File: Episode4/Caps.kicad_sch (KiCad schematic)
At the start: 192 parts

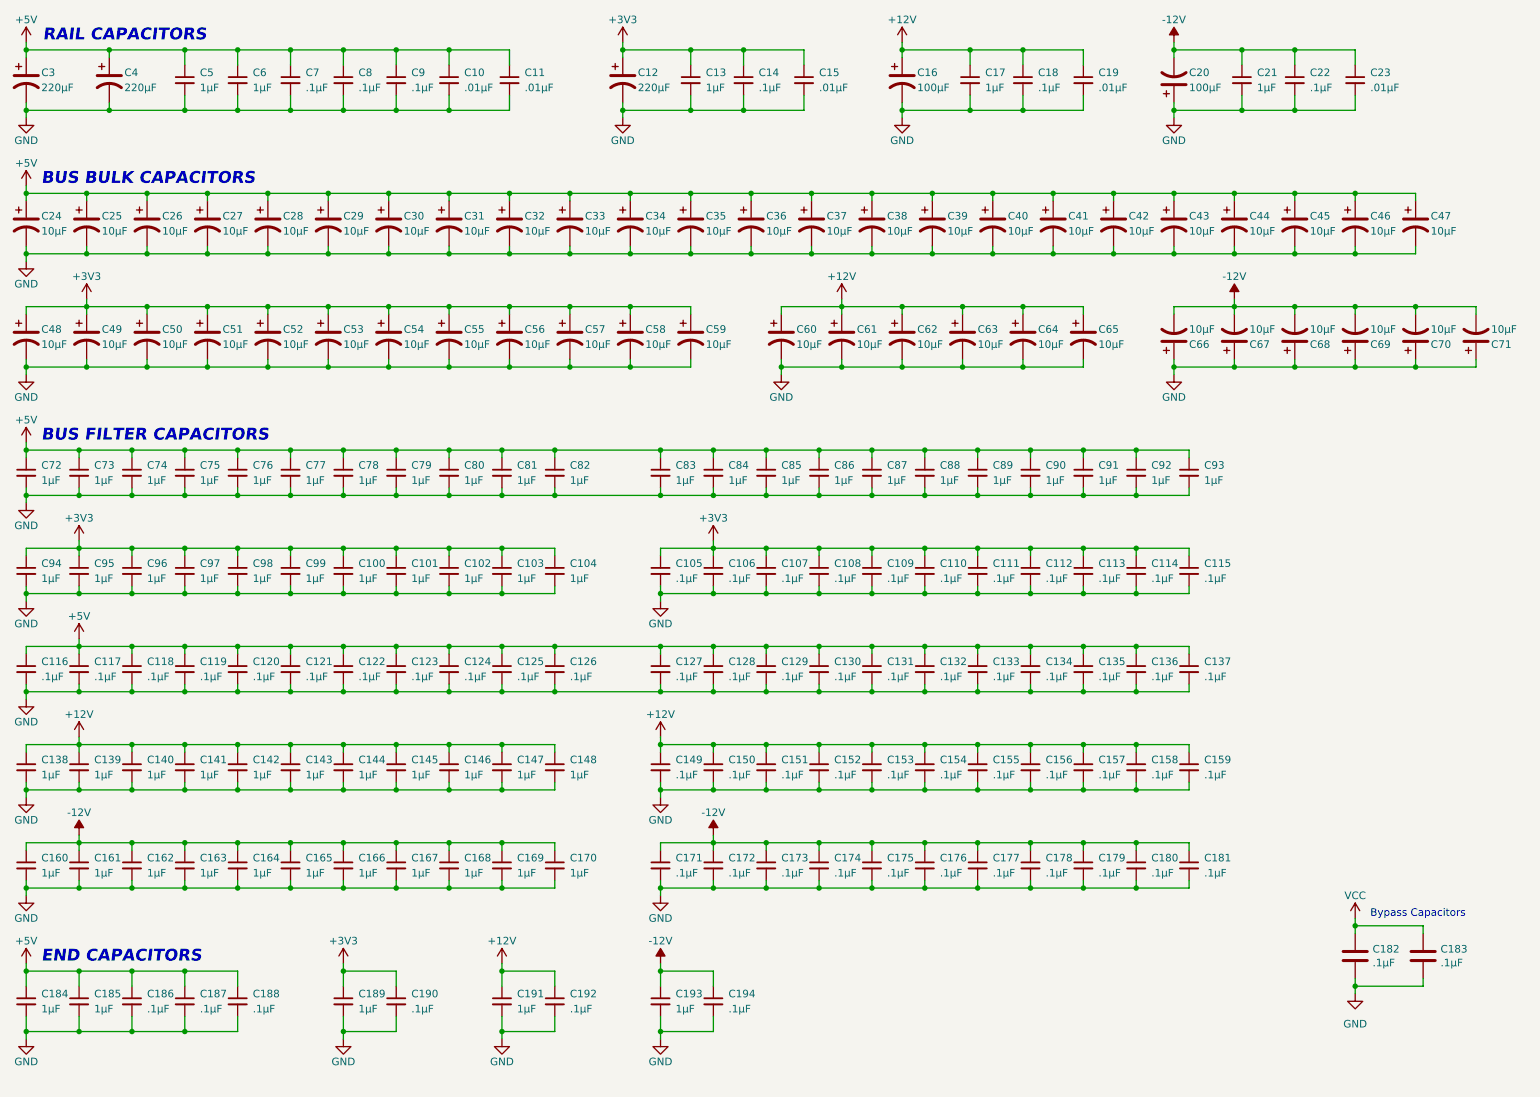
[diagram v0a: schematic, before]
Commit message: Finished the backplane
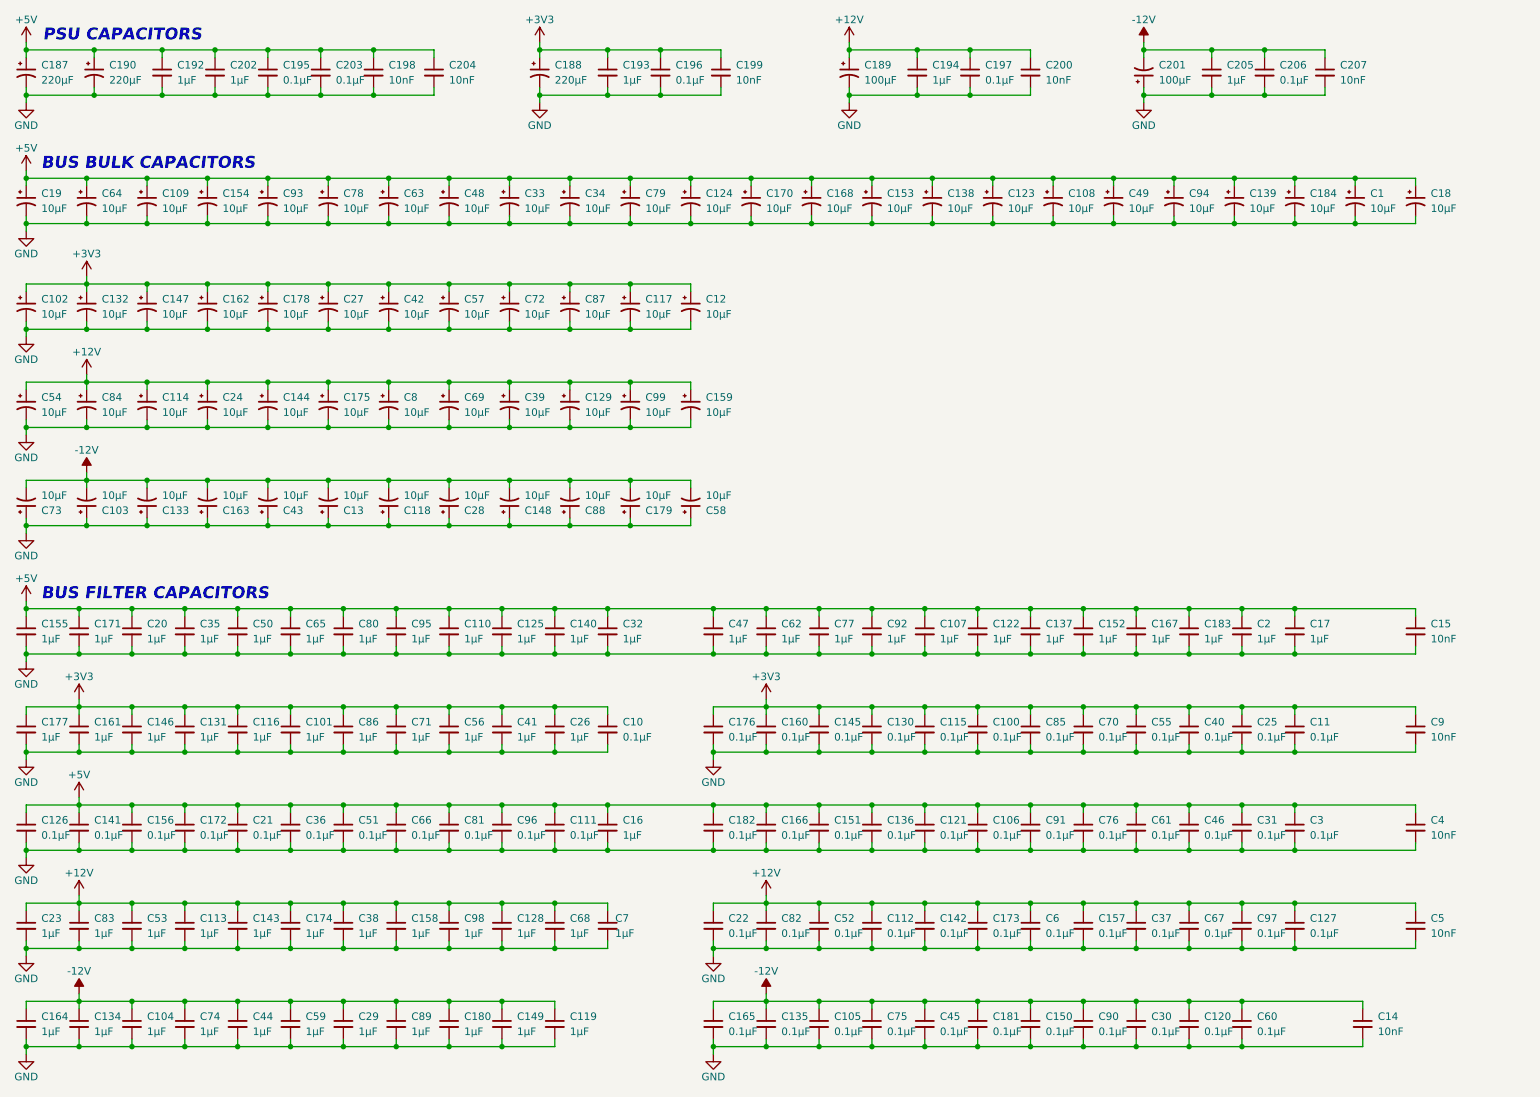
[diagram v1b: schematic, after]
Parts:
- removed C144, C145, C146, C147, C148, C165, C166, C167, C168, C169, C170, C191, C193: 1µF, Capacitor_SMD:C_0805_2012Metric_Pad1.18x1.45mm_HandSolder, symbol Device:C_Small
- removed C155, C156, C159, C171, C172, C173, C174, C175, C176, C188, C192, C194, C8: .1µF, Capacitor_SMD:C_0805_2012Metric_Pad1.18x1.45mm_HandSolder, symbol Device:C_Small
- removed C182, C183: .1µF, Capacitor_SMD:C_0805_2012Metric_Pad1.18x1.45mm_HandSolder, symbol Device:C
- added C118, C129, C148, C159, C179, C28, C39, C58, C69, C8, C88, C99: 10µF, Capacitor_SMD:CP_Elec_4x5.8, symbol Device:C_Polarized_Small_US
- added C119, C128, C149, C180, C29, C38, C59, C68, C7, C89, C98: 1µF, Capacitor_SMD:C_0805_2012Metric_Pad1.18x1.45mm_HandSolder, symbol Device:C_Small
- added C120, C127, C150, C181, C30, C37, C6, C60, C67, C90, C97: 0.1µF, Capacitor_SMD:C_0805_2012Metric_Pad1.18x1.45mm_HandSolder, symbol Device:C_Small
- added C14, C15, C4, C5, C9: 10nF, Capacitor_SMD:C_0805_2012Metric_Pad1.18x1.45mm_HandSolder, symbol Device:C_Small
- C1: renamed from C46; symbol Device:C_Polarized_US -> Device:C_Polarized_Small_US
- C10: renamed from C187; value .1µF -> 0.1µF; Manufacturer_Name Samsung Electro-Mechanics -> TAIYO YUDEN; Manufacturer_Part_Number CL21B104KBFNNNG -> MCASU21GSB7104KTNA01
- C100: renamed from C110; value .1µF -> 0.1µF; Manufacturer_Name Samsung Electro-Mechanics -> TAIYO YUDEN; Manufacturer_Part_Number CL21B104KBFNNNG -> MCASU21GSB7104KTNA01
- C101: renamed from C99; Manufacturer_Name Samsung Electro-Mechanics -> TAIYO YUDEN; Manufacturer_Part_Number CL21B105KBFNNNG -> MCASU21GSB7105KTNA01
- C102: renamed from C48; symbol Device:C_Polarized_US -> Device:C_Polarized_Small_US
- C103: renamed from C67; symbol Device:C_Polarized_US -> Device:C_Polarized_Small_US
- C104: renamed from C162; Manufacturer_Name Samsung Electro-Mechanics -> TAIYO YUDEN; Manufacturer_Part_Number CL21B105KBFNNNG -> MCASU21GSB7105KTNA01
- C105: renamed from C179; value .1µF -> 0.1µF; Manufacturer_Name Samsung Electro-Mechanics -> TAIYO YUDEN; Manufacturer_Part_Number CL21B104KBFNNNG -> MCASU21GSB7104KTNA01
- C106: renamed from C132; value .1µF -> 0.1µF; Manufacturer_Name Samsung Electro-Mechanics -> TAIYO YUDEN; Manufacturer_Part_Number CL21B104KBFNNNG -> MCASU21GSB7104KTNA01
- C107: renamed from C88; Manufacturer_Name Samsung Electro-Mechanics -> TAIYO YUDEN; Manufacturer_Part_Number CL21B105KBFNNNG -> MCASU21GSB7105KTNA01
- C108: renamed from C41; symbol Device:C_Polarized_US -> Device:C_Polarized_Small_US
- C109: renamed from C26; symbol Device:C_Polarized_US -> Device:C_Polarized_Small_US
- C11: renamed from C186; value .1µF -> 0.1µF; Manufacturer_Name Samsung Electro-Mechanics -> TAIYO YUDEN; Manufacturer_Part_Number CL21B104KBFNNNG -> MCASU21GSB7104KTNA01
- C110: renamed from C80; Manufacturer_Name Samsung Electro-Mechanics -> TAIYO YUDEN; Manufacturer_Part_Number CL21B105KBFNNNG -> MCASU21GSB7105KTNA01
- C111: renamed from C126; value .1µF -> 0.1µF; Manufacturer_Name Samsung Electro-Mechanics -> TAIYO YUDEN; Manufacturer_Part_Number CL21B104KBFNNNG -> MCASU21GSB7104KTNA01
- C112: renamed from C152; value .1µF -> 0.1µF; Manufacturer_Name Samsung Electro-Mechanics -> TAIYO YUDEN; Manufacturer_Part_Number CL21B104KBFNNNG -> MCASU21GSB7104KTNA01
- C113: renamed from C141; Manufacturer_Name Samsung Electro-Mechanics -> TAIYO YUDEN; Manufacturer_Part_Number CL21B105KBFNNNG -> MCASU21GSB7105KTNA01
- C114: renamed from C62; symbol Device:C_Polarized_US -> Device:C_Polarized_Small_US
- C115: renamed from C109; value .1µF -> 0.1µF; Manufacturer_Name Samsung Electro-Mechanics -> TAIYO YUDEN; Manufacturer_Part_Number CL21B104KBFNNNG -> MCASU21GSB7104KTNA01
- C116: renamed from C98; Manufacturer_Name Samsung Electro-Mechanics -> TAIYO YUDEN; Manufacturer_Part_Number CL21B105KBFNNNG -> MCASU21GSB7105KTNA01
- C117: renamed from C58; symbol Device:C_Polarized_US -> Device:C_Polarized_Small_US
- C12: renamed from C59; symbol Device:C_Polarized_US -> Device:C_Polarized_Small_US
- C121: renamed from C131; value .1µF -> 0.1µF; Manufacturer_Name Samsung Electro-Mechanics -> TAIYO YUDEN; Manufacturer_Part_Number CL21B104KBFNNNG -> MCASU21GSB7104KTNA01
- C122: renamed from C89; Manufacturer_Name Samsung Electro-Mechanics -> TAIYO YUDEN; Manufacturer_Part_Number CL21B105KBFNNNG -> MCASU21GSB7105KTNA01
- C123: renamed from C40; symbol Device:C_Polarized_US -> Device:C_Polarized_Small_US
- C124: renamed from C35; symbol Device:C_Polarized_US -> Device:C_Polarized_Small_US
- C125: renamed from C81; Manufacturer_Name Samsung Electro-Mechanics -> TAIYO YUDEN; Manufacturer_Part_Number CL21B105KBFNNNG -> MCASU21GSB7105KTNA01
- C126: renamed from C116; value .1µF -> 0.1µF; Manufacturer_Name Samsung Electro-Mechanics -> TAIYO YUDEN; Manufacturer_Part_Number CL21B104KBFNNNG -> MCASU21GSB7104KTNA01
- C13: renamed from C71; symbol Device:C_Polarized_US -> Device:C_Polarized_Small_US
- C130: renamed from C108; value .1µF -> 0.1µF; Manufacturer_Name Samsung Electro-Mechanics -> TAIYO YUDEN; Manufacturer_Part_Number CL21B104KBFNNNG -> MCASU21GSB7104KTNA01
- C131: renamed from C97; Manufacturer_Name Samsung Electro-Mechanics -> TAIYO YUDEN; Manufacturer_Part_Number CL21B105KBFNNNG -> MCASU21GSB7105KTNA01
- C132: renamed from C49; symbol Device:C_Polarized_US -> Device:C_Polarized_Small_US
- C133: renamed from C68; symbol Device:C_Polarized_US -> Device:C_Polarized_Small_US
- C134: renamed from C161; Manufacturer_Name Samsung Electro-Mechanics -> TAIYO YUDEN; Manufacturer_Part_Number CL21B105KBFNNNG -> MCASU21GSB7105KTNA01
- C135: renamed from C178; value .1µF -> 0.1µF; Manufacturer_Name Samsung Electro-Mechanics -> TAIYO YUDEN; Manufacturer_Part_Number CL21B104KBFNNNG -> MCASU21GSB7104KTNA01
- C136: renamed from C130; value .1µF -> 0.1µF; Manufacturer_Name Samsung Electro-Mechanics -> TAIYO YUDEN; Manufacturer_Part_Number CL21B104KBFNNNG -> MCASU21GSB7104KTNA01
- C137: renamed from C90; Manufacturer_Name Samsung Electro-Mechanics -> TAIYO YUDEN; Manufacturer_Part_Number CL21B105KBFNNNG -> MCASU21GSB7105KTNA01
- C138: renamed from C39; symbol Device:C_Polarized_US -> Device:C_Polarized_Small_US
- C139: renamed from C44; symbol Device:C_Polarized_US -> Device:C_Polarized_Small_US
- C140: renamed from C82; Manufacturer_Name Samsung Electro-Mechanics -> TAIYO YUDEN; Manufacturer_Part_Number CL21B105KBFNNNG -> MCASU21GSB7105KTNA01
- C141: renamed from C117; value .1µF -> 0.1µF; Manufacturer_Name Samsung Electro-Mechanics -> TAIYO YUDEN; Manufacturer_Part_Number CL21B104KBFNNNG -> MCASU21GSB7104KTNA01
- C142: renamed from C153; value .1µF -> 0.1µF; Manufacturer_Name Samsung Electro-Mechanics -> TAIYO YUDEN; Manufacturer_Part_Number CL21B104KBFNNNG -> MCASU21GSB7104KTNA01
- C143: renamed from C142; Manufacturer_Name Samsung Electro-Mechanics -> TAIYO YUDEN; Manufacturer_Part_Number CL21B105KBFNNNG -> MCASU21GSB7105KTNA01
- C144: renamed from C64; symbol Device:C_Polarized_US -> Device:C_Polarized_Small_US
- C145: renamed from C107; value .1µF -> 0.1µF; Manufacturer_Name Samsung Electro-Mechanics -> TAIYO YUDEN; Manufacturer_Part_Number CL21B104KBFNNNG -> MCASU21GSB7104KTNA01
- C146: renamed from C96; Manufacturer_Name Samsung Electro-Mechanics -> TAIYO YUDEN; Manufacturer_Part_Number CL21B105KBFNNNG -> MCASU21GSB7105KTNA01
- C147: renamed from C50; symbol Device:C_Polarized_US -> Device:C_Polarized_Small_US
- C151: renamed from C129; value .1µF -> 0.1µF; Manufacturer_Name Samsung Electro-Mechanics -> TAIYO YUDEN; Manufacturer_Part_Number CL21B104KBFNNNG -> MCASU21GSB7104KTNA01
- C152: renamed from C91; Manufacturer_Name Samsung Electro-Mechanics -> TAIYO YUDEN; Manufacturer_Part_Number CL21B105KBFNNNG -> MCASU21GSB7105KTNA01
- C153: renamed from C38; symbol Device:C_Polarized_US -> Device:C_Polarized_Small_US
- C154: renamed from C27; symbol Device:C_Polarized_US -> Device:C_Polarized_Small_US
- C155: renamed from C72; Manufacturer_Name Samsung Electro-Mechanics -> TAIYO YUDEN; Manufacturer_Part_Number CL21B105KBFNNNG -> MCASU21GSB7105KTNA01
- C156: renamed from C118; value .1µF -> 0.1µF; Manufacturer_Name Samsung Electro-Mechanics -> TAIYO YUDEN; Manufacturer_Part_Number CL21B104KBFNNNG -> MCASU21GSB7104KTNA01
- C157: value .1µF -> 0.1µF; Manufacturer_Name Samsung Electro-Mechanics -> TAIYO YUDEN; Manufacturer_Part_Number CL21B104KBFNNNG -> MCASU21GSB7104KTNA01
- C158: value .1µF -> 1µF; Manufacturer_Name Samsung Electro-Mechanics -> TAIYO YUDEN; Manufacturer_Part_Number CL21B104KBFNNNG -> MCASU21GSB7105KTNA01
- C16: renamed from C189; Manufacturer_Name Samsung Electro-Mechanics -> TAIYO YUDEN; Manufacturer_Part_Number CL21B105KBFNNNG -> MCASU21GSB7105KTNA01
- C160: renamed from C106; value .1µF -> 0.1µF; Manufacturer_Name Samsung Electro-Mechanics -> TAIYO YUDEN; Manufacturer_Part_Number CL21B104KBFNNNG -> MCASU21GSB7104KTNA01
- C161: renamed from C95; Manufacturer_Name Samsung Electro-Mechanics -> TAIYO YUDEN; Manufacturer_Part_Number CL21B105KBFNNNG -> MCASU21GSB7105KTNA01
- C162: renamed from C51; symbol Device:C_Polarized_US -> Device:C_Polarized_Small_US
- C163: renamed from C69; symbol Device:C_Polarized_US -> Device:C_Polarized_Small_US
- C164: renamed from C160; Manufacturer_Name Samsung Electro-Mechanics -> TAIYO YUDEN; Manufacturer_Part_Number CL21B105KBFNNNG -> MCASU21GSB7105KTNA01
- C165: renamed from C177; value .1µF -> 0.1µF; Manufacturer_Name Samsung Electro-Mechanics -> TAIYO YUDEN; Manufacturer_Part_Number CL21B104KBFNNNG -> MCASU21GSB7104KTNA01
- C166: renamed from C128; value .1µF -> 0.1µF; Manufacturer_Name Samsung Electro-Mechanics -> TAIYO YUDEN; Manufacturer_Part_Number CL21B104KBFNNNG -> MCASU21GSB7104KTNA01
- C167: renamed from C92; Manufacturer_Name Samsung Electro-Mechanics -> TAIYO YUDEN; Manufacturer_Part_Number CL21B105KBFNNNG -> MCASU21GSB7105KTNA01
- C168: renamed from C37; symbol Device:C_Polarized_US -> Device:C_Polarized_Small_US
- C17: renamed from C185; Manufacturer_Name Samsung Electro-Mechanics -> TAIYO YUDEN; Manufacturer_Part_Number CL21B105KBFNNNG -> MCASU21GSB7105KTNA01
- C170: renamed from C36; symbol Device:C_Polarized_US -> Device:C_Polarized_Small_US
- C171: renamed from C73; Manufacturer_Name Samsung Electro-Mechanics -> TAIYO YUDEN; Manufacturer_Part_Number CL21B105KBFNNNG -> MCASU21GSB7105KTNA01
- C172: renamed from C119; value .1µF -> 0.1µF; Manufacturer_Name Samsung Electro-Mechanics -> TAIYO YUDEN; Manufacturer_Part_Number CL21B104KBFNNNG -> MCASU21GSB7104KTNA01
- C173: renamed from C154; value .1µF -> 0.1µF; Manufacturer_Name Samsung Electro-Mechanics -> TAIYO YUDEN; Manufacturer_Part_Number CL21B104KBFNNNG -> MCASU21GSB7104KTNA01
- C174: renamed from C143; Manufacturer_Name Samsung Electro-Mechanics -> TAIYO YUDEN; Manufacturer_Part_Number CL21B105KBFNNNG -> MCASU21GSB7105KTNA01
- C175: renamed from C65; symbol Device:C_Polarized_US -> Device:C_Polarized_Small_US
- C176: renamed from C105; value .1µF -> 0.1µF; Manufacturer_Name Samsung Electro-Mechanics -> TAIYO YUDEN; Manufacturer_Part_Number CL21B104KBFNNNG -> MCASU21GSB7104KTNA01
- C177: renamed from C94; Manufacturer_Name Samsung Electro-Mechanics -> TAIYO YUDEN; Manufacturer_Part_Number CL21B105KBFNNNG -> MCASU21GSB7105KTNA01
- C178: renamed from C52; symbol Device:C_Polarized_US -> Device:C_Polarized_Small_US
- C18: renamed from C47; symbol Device:C_Polarized_US -> Device:C_Polarized_Small_US
- C182: renamed from C127; value .1µF -> 0.1µF; Manufacturer_Name Samsung Electro-Mechanics -> TAIYO YUDEN; Manufacturer_Part_Number CL21B104KBFNNNG -> MCASU21GSB7104KTNA01
- C183: renamed from C93; Manufacturer_Name Samsung Electro-Mechanics -> TAIYO YUDEN; Manufacturer_Part_Number CL21B105KBFNNNG -> MCASU21GSB7105KTNA01
- C184: renamed from C45; symbol Device:C_Polarized_US -> Device:C_Polarized_Small_US
- C187: renamed from C3; symbol Device:C_Polarized_US -> Device:C_Polarized_Small_US
- C188: renamed from C12; symbol Device:C_Polarized_US -> Device:C_Polarized_Small_US
- C189: renamed from C16; symbol Device:C_Polarized_US -> Device:C_Polarized_Small_US
- C19: renamed from C24; symbol Device:C_Polarized_US -> Device:C_Polarized_Small_US
- C190: renamed from C4; symbol Device:C_Polarized_US -> Device:C_Polarized_Small_US
- C192: renamed from C5; Manufacturer_Name Samsung Electro-Mechanics -> TAIYO YUDEN; Manufacturer_Part_Number CL21B105KBFNNNG -> MCASU21GSB7105KTNA01
- C193: renamed from C13; Manufacturer_Name Samsung Electro-Mechanics -> TAIYO YUDEN; Manufacturer_Part_Number CL21B105KBFNNNG -> MCASU21GSB7105KTNA01
- C194: renamed from C17; Manufacturer_Name Samsung Electro-Mechanics -> TAIYO YUDEN; Manufacturer_Part_Number CL21B105KBFNNNG -> MCASU21GSB7105KTNA01
- C195: renamed from C7; value .1µF -> 0.1µF; Manufacturer_Name Samsung Electro-Mechanics -> TAIYO YUDEN; Manufacturer_Part_Number CL21B104KBFNNNG -> MCASU21GSB7104KTNA01
- C196: renamed from C14; value .1µF -> 0.1µF; Manufacturer_Name Samsung Electro-Mechanics -> TAIYO YUDEN; Manufacturer_Part_Number CL21B104KBFNNNG -> MCASU21GSB7104KTNA01
- C197: renamed from C18; value .1µF -> 0.1µF; Manufacturer_Name Samsung Electro-Mechanics -> TAIYO YUDEN; Manufacturer_Part_Number CL21B104KBFNNNG -> MCASU21GSB7104KTNA01
- C198: renamed from C10; value .01µF -> 10nF; Manufacturer_Name Samsung Electro-Mechanics -> TAIYO YUDEN; Manufacturer_Part_Number CL21B103KBCNNNC -> MCASU21GSB7103KTNA01
- C199: renamed from C15; value .01µF -> 10nF; Manufacturer_Name Samsung Electro-Mechanics -> TAIYO YUDEN; Manufacturer_Part_Number CL21B103KBCNNNC -> MCASU21GSB7103KTNA01
- C2: renamed from C184; Manufacturer_Name Samsung Electro-Mechanics -> TAIYO YUDEN; Manufacturer_Part_Number CL21B105KBFNNNG -> MCASU21GSB7105KTNA01
- C20: renamed from C74; Manufacturer_Name Samsung Electro-Mechanics -> TAIYO YUDEN; Manufacturer_Part_Number CL21B105KBFNNNG -> MCASU21GSB7105KTNA01
- C200: renamed from C19; value .01µF -> 10nF; Manufacturer_Name Samsung Electro-Mechanics -> TAIYO YUDEN; Manufacturer_Part_Number CL21B103KBCNNNC -> MCASU21GSB7103KTNA01
- C201: renamed from C20; symbol Device:C_Polarized_US -> Device:C_Polarized_Small_US
- C202: renamed from C6; Manufacturer_Name Samsung Electro-Mechanics -> TAIYO YUDEN; Manufacturer_Part_Number CL21B105KBFNNNG -> MCASU21GSB7105KTNA01
- C203: renamed from C9; value .1µF -> 0.1µF; Manufacturer_Name Samsung Electro-Mechanics -> TAIYO YUDEN; Manufacturer_Part_Number CL21B104KBFNNNG -> MCASU21GSB7104KTNA01
- C204: renamed from C11; value .01µF -> 10nF; Manufacturer_Name Samsung Electro-Mechanics -> TAIYO YUDEN; Manufacturer_Part_Number CL21B103KBCNNNC -> MCASU21GSB7103KTNA01
- C205: renamed from C21; Manufacturer_Name Samsung Electro-Mechanics -> TAIYO YUDEN; Manufacturer_Part_Number CL21B105KBFNNNG -> MCASU21GSB7105KTNA01
- C206: renamed from C22; value .1µF -> 0.1µF; Manufacturer_Name Samsung Electro-Mechanics -> TAIYO YUDEN; Manufacturer_Part_Number CL21B104KBFNNNG -> MCASU21GSB7104KTNA01
- C207: renamed from C23; value .01µF -> 10nF; Manufacturer_Name Samsung Electro-Mechanics -> TAIYO YUDEN; Manufacturer_Part_Number CL21B103KBCNNNC -> MCASU21GSB7103KTNA01
- C21: renamed from C120; value .1µF -> 0.1µF; Manufacturer_Name Samsung Electro-Mechanics -> TAIYO YUDEN; Manufacturer_Part_Number CL21B104KBFNNNG -> MCASU21GSB7104KTNA01
- C22: renamed from C149; value .1µF -> 0.1µF; Manufacturer_Name Samsung Electro-Mechanics -> TAIYO YUDEN; Manufacturer_Part_Number CL21B104KBFNNNG -> MCASU21GSB7104KTNA01
- C23: renamed from C138; Manufacturer_Name Samsung Electro-Mechanics -> TAIYO YUDEN; Manufacturer_Part_Number CL21B105KBFNNNG -> MCASU21GSB7105KTNA01
- C24: renamed from C63; symbol Device:C_Polarized_US -> Device:C_Polarized_Small_US
- C25: renamed from C115; value .1µF -> 0.1µF; Manufacturer_Name Samsung Electro-Mechanics -> TAIYO YUDEN; Manufacturer_Part_Number CL21B104KBFNNNG -> MCASU21GSB7104KTNA01
- C26: renamed from C104; Manufacturer_Name Samsung Electro-Mechanics -> TAIYO YUDEN; Manufacturer_Part_Number CL21B105KBFNNNG -> MCASU21GSB7105KTNA01
- C27: renamed from C53; symbol Device:C_Polarized_US -> Device:C_Polarized_Small_US
- C3: renamed from C190; value .1µF -> 0.1µF; Manufacturer_Name Samsung Electro-Mechanics -> TAIYO YUDEN; Manufacturer_Part_Number CL21B104KBFNNNG -> MCASU21GSB7104KTNA01
- C31: renamed from C137; value .1µF -> 0.1µF; Manufacturer_Name Samsung Electro-Mechanics -> TAIYO YUDEN; Manufacturer_Part_Number CL21B104KBFNNNG -> MCASU21GSB7104KTNA01
- C32: renamed from C83; Manufacturer_Name Samsung Electro-Mechanics -> TAIYO YUDEN; Manufacturer_Part_Number CL21B105KBFNNNG -> MCASU21GSB7105KTNA01
- C33: renamed from C32; symbol Device:C_Polarized_US -> Device:C_Polarized_Small_US
- C34: renamed from C33; symbol Device:C_Polarized_US -> Device:C_Polarized_Small_US
- C35: renamed from C75; Manufacturer_Name Samsung Electro-Mechanics -> TAIYO YUDEN; Manufacturer_Part_Number CL21B105KBFNNNG -> MCASU21GSB7105KTNA01
- C36: renamed from C121; value .1µF -> 0.1µF; Manufacturer_Name Samsung Electro-Mechanics -> TAIYO YUDEN; Manufacturer_Part_Number CL21B104KBFNNNG -> MCASU21GSB7104KTNA01
- C40: renamed from C114; value .1µF -> 0.1µF; Manufacturer_Name Samsung Electro-Mechanics -> TAIYO YUDEN; Manufacturer_Part_Number CL21B104KBFNNNG -> MCASU21GSB7104KTNA01
- C41: renamed from C103; Manufacturer_Name Samsung Electro-Mechanics -> TAIYO YUDEN; Manufacturer_Part_Number CL21B105KBFNNNG -> MCASU21GSB7105KTNA01
- C42: renamed from C54; symbol Device:C_Polarized_US -> Device:C_Polarized_Small_US
- C43: renamed from C70; symbol Device:C_Polarized_US -> Device:C_Polarized_Small_US
- C44: renamed from C164; Manufacturer_Name Samsung Electro-Mechanics -> TAIYO YUDEN; Manufacturer_Part_Number CL21B105KBFNNNG -> MCASU21GSB7105KTNA01
- C45: renamed from C181; value .1µF -> 0.1µF; Manufacturer_Name Samsung Electro-Mechanics -> TAIYO YUDEN; Manufacturer_Part_Number CL21B104KBFNNNG -> MCASU21GSB7104KTNA01
- C46: renamed from C136; value .1µF -> 0.1µF; Manufacturer_Name Samsung Electro-Mechanics -> TAIYO YUDEN; Manufacturer_Part_Number CL21B104KBFNNNG -> MCASU21GSB7104KTNA01
- C47: renamed from C84; Manufacturer_Name Samsung Electro-Mechanics -> TAIYO YUDEN; Manufacturer_Part_Number CL21B105KBFNNNG -> MCASU21GSB7105KTNA01
- C48: renamed from C31; symbol Device:C_Polarized_US -> Device:C_Polarized_Small_US
- C49: renamed from C42; symbol Device:C_Polarized_US -> Device:C_Polarized_Small_US
- C50: renamed from C76; Manufacturer_Name Samsung Electro-Mechanics -> TAIYO YUDEN; Manufacturer_Part_Number CL21B105KBFNNNG -> MCASU21GSB7105KTNA01
- C51: renamed from C122; value .1µF -> 0.1µF; Manufacturer_Name Samsung Electro-Mechanics -> TAIYO YUDEN; Manufacturer_Part_Number CL21B104KBFNNNG -> MCASU21GSB7104KTNA01
- C52: renamed from C151; value .1µF -> 0.1µF; Manufacturer_Name Samsung Electro-Mechanics -> TAIYO YUDEN; Manufacturer_Part_Number CL21B104KBFNNNG -> MCASU21GSB7104KTNA01
- C53: renamed from C140; Manufacturer_Name Samsung Electro-Mechanics -> TAIYO YUDEN; Manufacturer_Part_Number CL21B105KBFNNNG -> MCASU21GSB7105KTNA01
- C54: renamed from C60; symbol Device:C_Polarized_US -> Device:C_Polarized_Small_US
- C55: renamed from C113; value .1µF -> 0.1µF; Manufacturer_Name Samsung Electro-Mechanics -> TAIYO YUDEN; Manufacturer_Part_Number CL21B104KBFNNNG -> MCASU21GSB7104KTNA01
- C56: renamed from C102; Manufacturer_Name Samsung Electro-Mechanics -> TAIYO YUDEN; Manufacturer_Part_Number CL21B105KBFNNNG -> MCASU21GSB7105KTNA01
- C57: renamed from C55; symbol Device:C_Polarized_US -> Device:C_Polarized_Small_US
- C61: renamed from C135; value .1µF -> 0.1µF; Manufacturer_Name Samsung Electro-Mechanics -> TAIYO YUDEN; Manufacturer_Part_Number CL21B104KBFNNNG -> MCASU21GSB7104KTNA01
- C62: renamed from C85; Manufacturer_Name Samsung Electro-Mechanics -> TAIYO YUDEN; Manufacturer_Part_Number CL21B105KBFNNNG -> MCASU21GSB7105KTNA01
- C63: renamed from C30; symbol Device:C_Polarized_US -> Device:C_Polarized_Small_US
- C64: renamed from C25; symbol Device:C_Polarized_US -> Device:C_Polarized_Small_US
- C65: renamed from C77; Manufacturer_Name Samsung Electro-Mechanics -> TAIYO YUDEN; Manufacturer_Part_Number CL21B105KBFNNNG -> MCASU21GSB7105KTNA01
- C66: renamed from C123; value .1µF -> 0.1µF; Manufacturer_Name Samsung Electro-Mechanics -> TAIYO YUDEN; Manufacturer_Part_Number CL21B104KBFNNNG -> MCASU21GSB7104KTNA01
- C70: renamed from C112; value .1µF -> 0.1µF; Manufacturer_Name Samsung Electro-Mechanics -> TAIYO YUDEN; Manufacturer_Part_Number CL21B104KBFNNNG -> MCASU21GSB7104KTNA01
- C71: renamed from C101; Manufacturer_Name Samsung Electro-Mechanics -> TAIYO YUDEN; Manufacturer_Part_Number CL21B105KBFNNNG -> MCASU21GSB7105KTNA01
- C72: renamed from C56; symbol Device:C_Polarized_US -> Device:C_Polarized_Small_US
- C73: renamed from C66; symbol Device:C_Polarized_US -> Device:C_Polarized_Small_US
- C74: renamed from C163; Manufacturer_Name Samsung Electro-Mechanics -> TAIYO YUDEN; Manufacturer_Part_Number CL21B105KBFNNNG -> MCASU21GSB7105KTNA01
- C75: renamed from C180; value .1µF -> 0.1µF; Manufacturer_Name Samsung Electro-Mechanics -> TAIYO YUDEN; Manufacturer_Part_Number CL21B104KBFNNNG -> MCASU21GSB7104KTNA01
- C76: renamed from C134; value .1µF -> 0.1µF; Manufacturer_Name Samsung Electro-Mechanics -> TAIYO YUDEN; Manufacturer_Part_Number CL21B104KBFNNNG -> MCASU21GSB7104KTNA01
- C77: renamed from C86; Manufacturer_Name Samsung Electro-Mechanics -> TAIYO YUDEN; Manufacturer_Part_Number CL21B105KBFNNNG -> MCASU21GSB7105KTNA01
- C78: renamed from C29; symbol Device:C_Polarized_US -> Device:C_Polarized_Small_US
- C79: renamed from C34; symbol Device:C_Polarized_US -> Device:C_Polarized_Small_US
- C80: renamed from C78; Manufacturer_Name Samsung Electro-Mechanics -> TAIYO YUDEN; Manufacturer_Part_Number CL21B105KBFNNNG -> MCASU21GSB7105KTNA01
- C81: renamed from C124; value .1µF -> 0.1µF; Manufacturer_Name Samsung Electro-Mechanics -> TAIYO YUDEN; Manufacturer_Part_Number CL21B104KBFNNNG -> MCASU21GSB7104KTNA01
- C82: renamed from C150; value .1µF -> 0.1µF; Manufacturer_Name Samsung Electro-Mechanics -> TAIYO YUDEN; Manufacturer_Part_Number CL21B104KBFNNNG -> MCASU21GSB7104KTNA01
- C83: renamed from C139; Manufacturer_Name Samsung Electro-Mechanics -> TAIYO YUDEN; Manufacturer_Part_Number CL21B105KBFNNNG -> MCASU21GSB7105KTNA01
- C84: renamed from C61; symbol Device:C_Polarized_US -> Device:C_Polarized_Small_US
- C85: renamed from C111; value .1µF -> 0.1µF; Manufacturer_Name Samsung Electro-Mechanics -> TAIYO YUDEN; Manufacturer_Part_Number CL21B104KBFNNNG -> MCASU21GSB7104KTNA01
- C86: renamed from C100; Manufacturer_Name Samsung Electro-Mechanics -> TAIYO YUDEN; Manufacturer_Part_Number CL21B105KBFNNNG -> MCASU21GSB7105KTNA01
- C87: renamed from C57; symbol Device:C_Polarized_US -> Device:C_Polarized_Small_US
- C91: renamed from C133; value .1µF -> 0.1µF; Manufacturer_Name Samsung Electro-Mechanics -> TAIYO YUDEN; Manufacturer_Part_Number CL21B104KBFNNNG -> MCASU21GSB7104KTNA01
- C92: renamed from C87; Manufacturer_Name Samsung Electro-Mechanics -> TAIYO YUDEN; Manufacturer_Part_Number CL21B105KBFNNNG -> MCASU21GSB7105KTNA01
- C93: renamed from C28; symbol Device:C_Polarized_US -> Device:C_Polarized_Small_US
- C94: renamed from C43; symbol Device:C_Polarized_US -> Device:C_Polarized_Small_US
- C95: renamed from C79; Manufacturer_Name Samsung Electro-Mechanics -> TAIYO YUDEN; Manufacturer_Part_Number CL21B105KBFNNNG -> MCASU21GSB7105KTNA01
- C96: renamed from C125; value .1µF -> 0.1µF; Manufacturer_Name Samsung Electro-Mechanics -> TAIYO YUDEN; Manufacturer_Part_Number CL21B104KBFNNNG -> MCASU21GSB7104KTNA01
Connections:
- net +12V: now also C127.1, C128.1, C129.1, C159.1, C37.1, C38.1, C39.1, C5.1, C6.1, C67.1, C68.1, C69.1, C7.1, C8.1, C97.1, C98.1, C99.1
- net +3V3: now also C10.1, C11.1, C9.1; no longer C16.1, C3.1
- net +5V: now also C16.1, C3.1, C15.1, C4.1; no longer C10.1, C11.1
- net -12V: now also C118.2, C119.1, C120.1, C14.1, C148.2, C149.1, C150.1, C179.2, C180.1, C181.1, C28.2, C29.1, C30.1, C58.2, C59.1, C60.1, C88.2, C89.1, C90.1
- net GND: now also C118.1, C119.2, C120.2, C127.2, C128.2, C129.2, C14.2, C148.1, C149.2, C15.2, C150.2, C159.2, C179.1, C180.2, C181.2, C28.1, C29.2, C30.2, C37.2, C38.2, C39.2, C4.2, C5.2, C58.1, C59.2, C6.2, C60.2, C67.2, C68.2, C69.2, C7.2, C8.2, C88.1, C89.2, C9.2, C90.2, C97.2, C98.2, C99.2
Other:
- note added: "PSU CAPACITORS"
- note removed: "Bypass Capacitors"
- note removed: "END CAPACITORS"
- note removed: "RAIL CAPACITORS"
- moved on the sheet: C1, C10, C100, C101, C102, C103, C104, C105, C106, C107, C108, C109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
